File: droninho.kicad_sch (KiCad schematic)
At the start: 19 parts, among them J1 M1, J2 M1, J3 M1, J4 M1, J5 Conn_01x02_Pin, Q1 SI2300, Q2 SI2300, Q3 SI2300, Q4 SI2300, U1 ESP32 Dev Kit, U2 MPU9250/6500

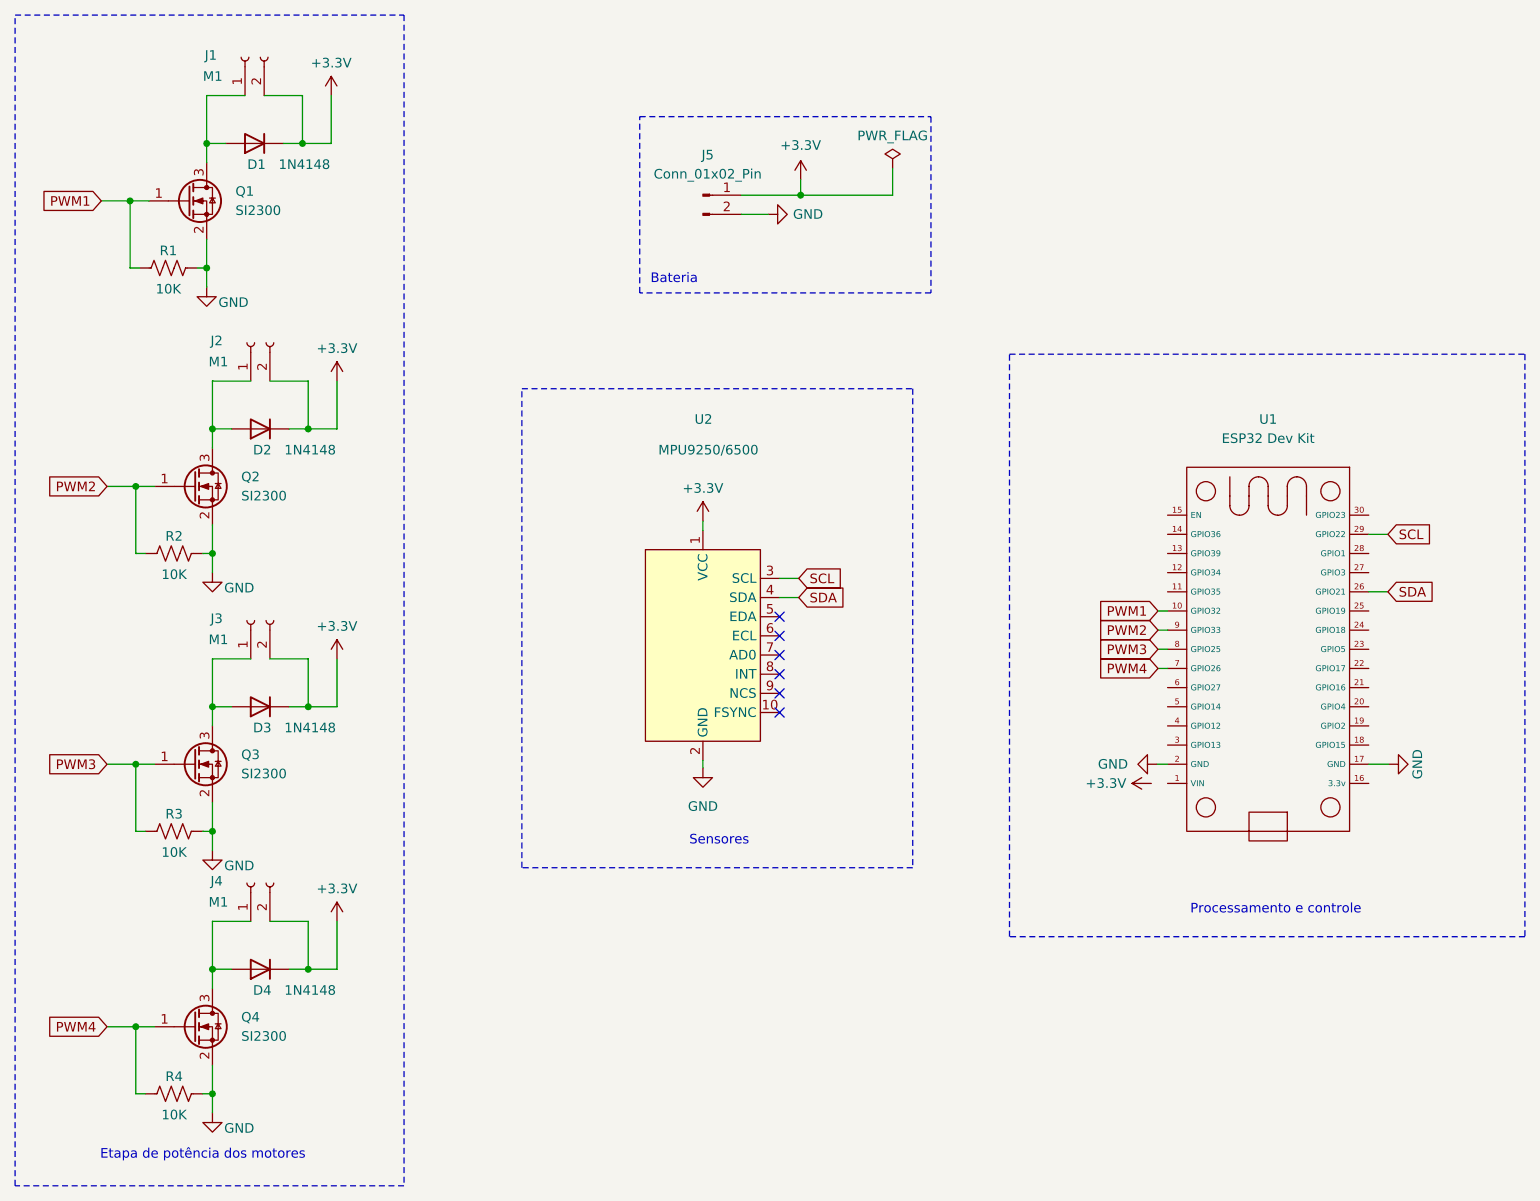
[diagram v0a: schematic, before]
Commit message: Electrical part finished
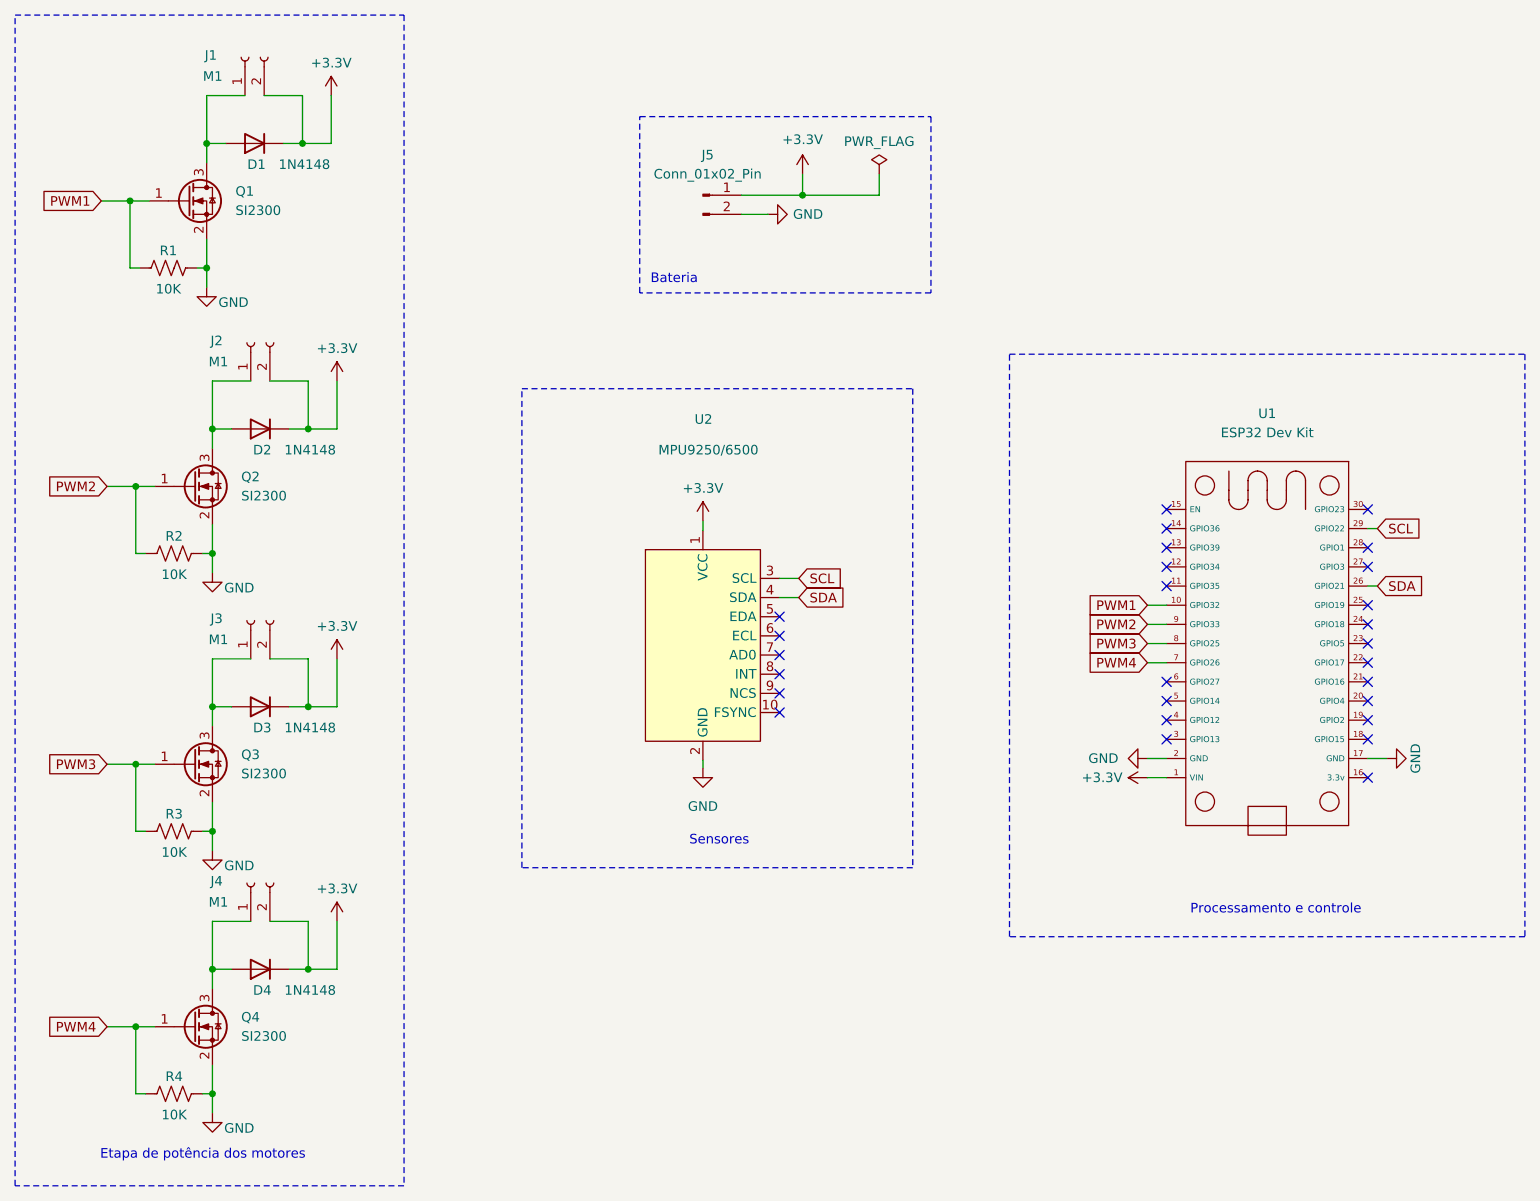
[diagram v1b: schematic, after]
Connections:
- net +3.3V: now also U1.1 (VIN)
- no-connect marks 6 -> 27
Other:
- moved on the sheet: U1
